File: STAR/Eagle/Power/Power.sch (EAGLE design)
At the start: 24 parts, among them J1 J30J-9J30, T1 750311838, U1 LT8300, U2 LT8330

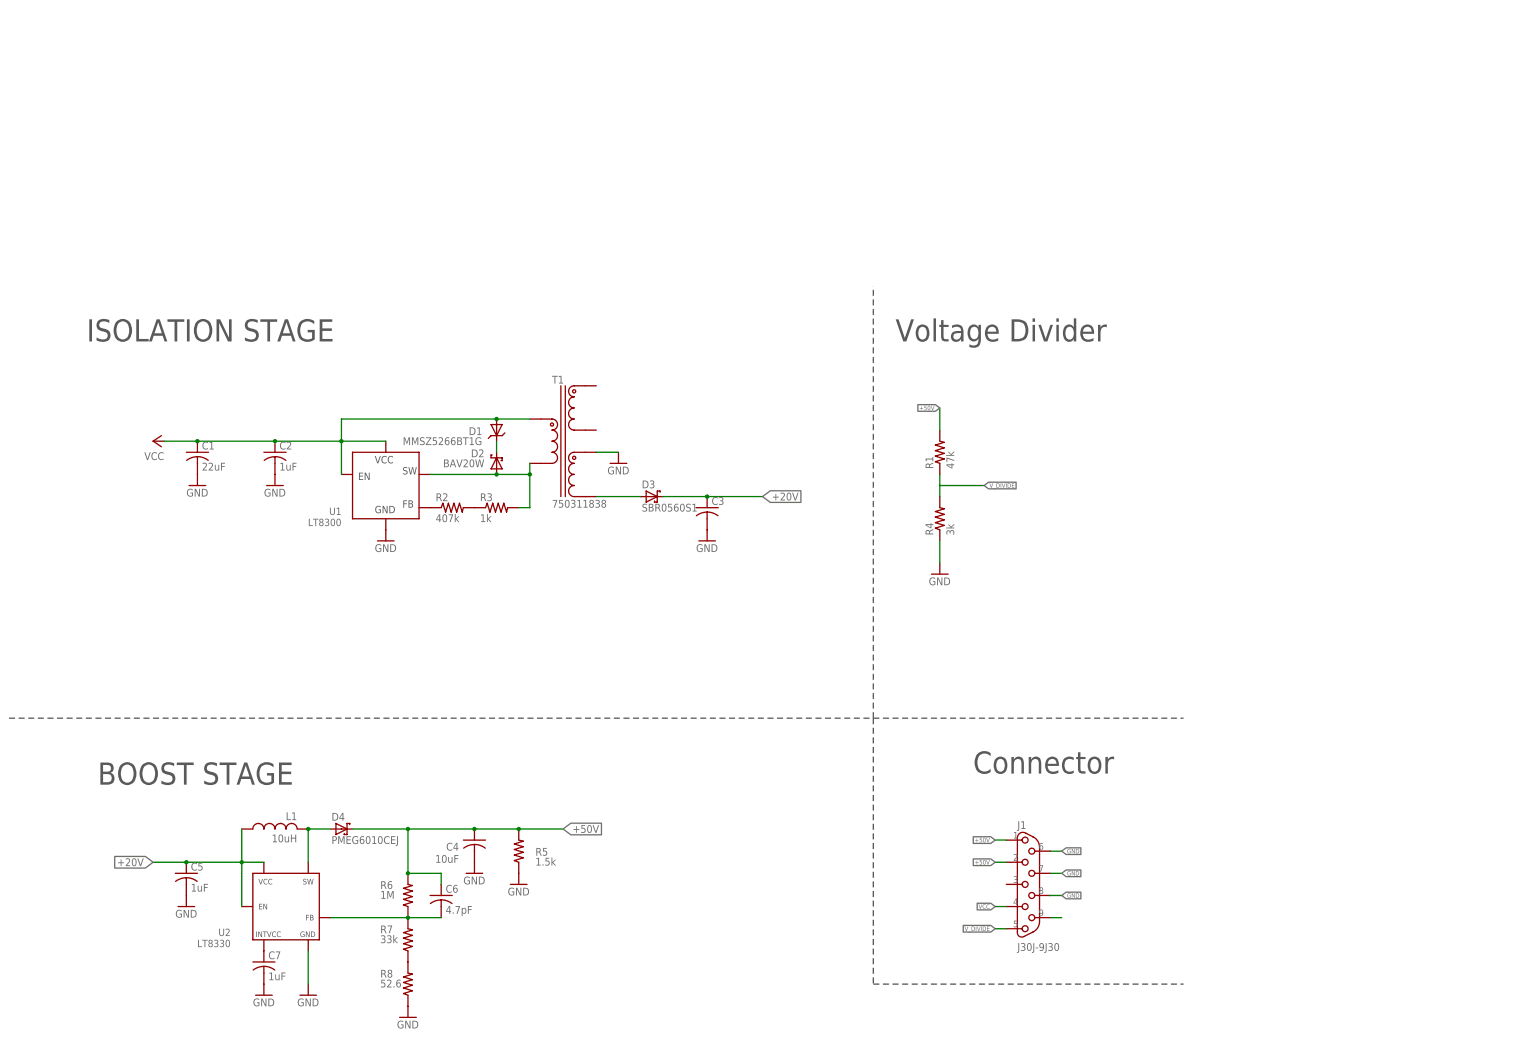
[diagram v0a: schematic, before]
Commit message: Power Board
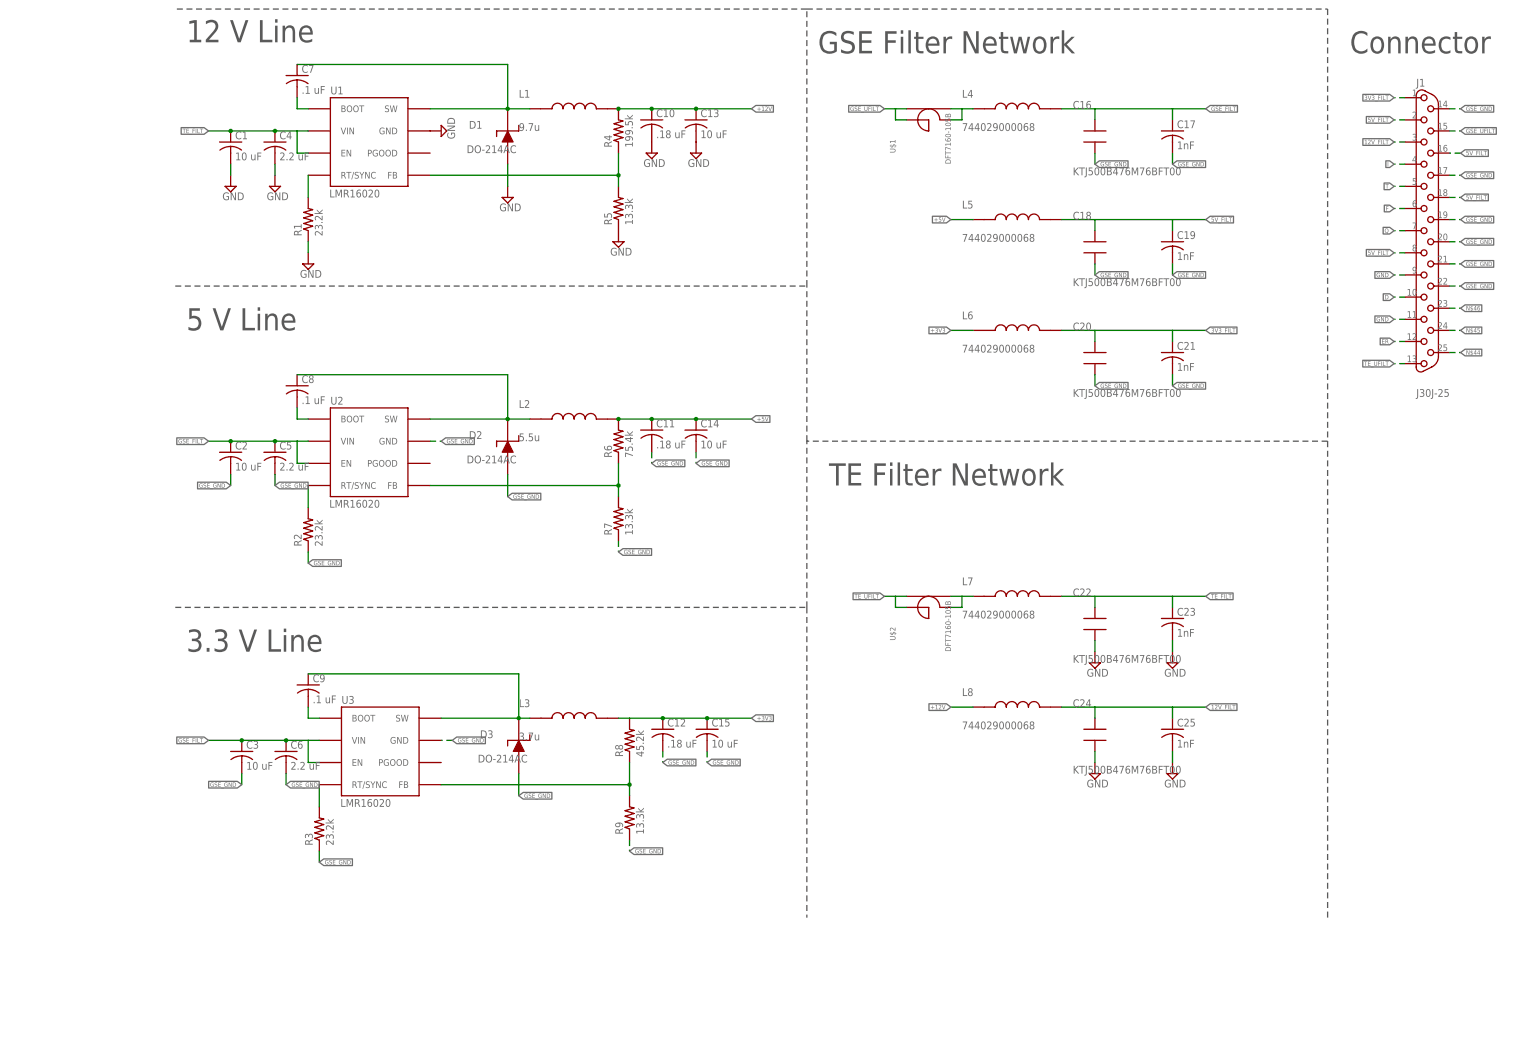
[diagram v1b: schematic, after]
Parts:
- removed D4: PMEG6010CEJ, AR_diode:SCHOTTKYSOD323
- removed T1: 750311838, AR_transformer:750311838
- added C10, C11, C12: .18 uF, resistor:C-USC0603
- added C13, C14, C15: 10 uF, resistor:C-USC0603
- added C16, C18, C20, C22, C24: KTJ500B476M76BFT00, Filtering:KTJ500B476M76BFT00
- added C17, C19, C21, C23, C25: 1nF, resistor:C-USC0603
- added C8, C9: .1 uF, resistor:C-USC0603
- added L2: 5.5u, Filtering:744325550
- added L3: 3.7u, Power:7443551370
- added L4, L5, L6, L7, L8: 744029000068, Filtering:744029000068
- added R9: 13.3k, resistor:R-US_R0603
- added U$1, U$2: DFT7160-105B, Filtering:DFT7160-105B
- added U3: LMR16020, HASP:LMR16020
- C1: value 22uF -> 10 uF; device AR_passives:CAPACITORC3025 -> resistor:C-USC1210
- C2: value 1uF -> 10 uF; device AR_passives:CAPACITORC0603 -> resistor:C-USC1210
- C3: value (none) -> 10 uF
- C4: value 10uF -> 2.2 uF; device AR_passives:CAPACITOR2-J-LEAD -> resistor:C-USC1210
- C5: value 1uF -> 2.2 uF; device AR_passives:CAPACITORC0603 -> resistor:C-USC1210
- C6: value 4.7pF -> 2.2 uF; device AR_passives:CAPACITORC0603 -> resistor:C-USC1210
- C7: value 1uF -> .1 uF; device AR_passives:CAPACITORC0603 -> resistor:C-USC0603
- D1: value MMSZ5266BT1G -> DO-214AC; device AR_diode:ZENERSOD123 -> HASP:DO-214AC
- D2: value BAV20W -> DO-214AC; device AR_diode:SCHOTTKYSOD323 -> HASP:DO-214AC
- D3: value SBR0560S1 -> DO-214AC; device AR_diode:SCHOTTKYSOD123 -> HASP:DO-214AC
- J1: value J30J-9J30 -> J30J-25; device CM_J30J:J30J-9J30 -> CM_J30J:J30J-25
- L1: value 10uH -> 9.7u; device AR_passives:INDUCTORPQ2614 -> Power:744314101
- R1: value 47k -> 23.2k; device resistor:R-US_R2512 -> resistor:R-US_R0603
- R2: value 407k -> 23.2k
- R3: value 1k -> 23.2k
- R4: value 3k -> 199.5k; device resistor:R-US_R2512 -> resistor:R-US_R0603
- R5: value 1.5k -> 13.3k; device resistor:R-US_R2512 -> resistor:R-US_R0603
- R6: value 1M -> 75.4k
- R7: value 33k -> 13.3k
- R8: value 52.6 -> 45.2k
- U1: value LT8300 -> LMR16020; device AR_IC:LT8300 -> HASP:LMR16020
- U2: value LT8330 -> LMR16020; device AR_IC:LT8330 -> HASP:LMR16020
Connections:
- removed net +20V: C3.1, C5.1, D3.C, L1.1, U2.EN, U2.VCC
- removed net +50V: C4.1, C6.1, D4.C, J1.1, J1.2, R1.2, R5.2, R6.2
- removed net N$11: R7.1, R8.2
- removed net VCC: C1.1, C2.1, D1.A, J1.4, T1.PA, U1.EN, U1.VCC
- removed net V_DIVIDE: J1.5, R1.1, R4.2
- new net +12V: C10.1, C13.1, L1.P$2, L8.P$1, R4.2
- new net +3V3: C12.1, C15.1, L3.P$2, L6.P$1, R8.2
- new net +5V: C11.1, C14.1, L2.P$2, L5.P$1, R6.2
- new net 12V_FILT: C24.P$1, C25.1, J1.3, L8.P$2
- new net 3V3_FILT: C20.P$1, C21.1, J1.1, L6.P$2
- new net 5V_FILT: C18.P$1, C19.1, J1.16, J1.18, J1.2, J1.8, L5.P$2
- new net D: J1.10
- new net ER: J1.12
- new net F: J1.6
- new net GSE_FILT: C16.P$1, C17.1, C2.1, C3.1, C5.1, C6.1, L4.P$2, U2.EN, U2.VIN, U3.EN, U3.VIN
- new net GSE_GND: C11.2, C12.2, C14.2, C15.2, C16.P$2, C17.2, C18.P$2, C19.2, C2.2, C20.P$2, C21.2, C3.2, C5.2, C6.2, D2.P$1, D3.P$1, J1.14, J1.17, J1.19, J1.20, J1.21, J1.22, R2.1, R3.1, R7.1, R9.1, U2.GND, U3.GND
- new net GSE_UFILT: J1.15, U$1.P$1, U$1.P$3
- new net I: J1.4
- new net N$14: C7.1, D1.P$2, L1.P$1, U1.SW
- new net N$27: R4.1, R5.2, U1.FB
- new net N$28: L4.P$1, U$1.P$2, U$1.P$4
- new net N$29: L7.P$1, U$2.P$2, U$2.P$4
- new net N$44: J1.25
- new net N$45: J1.24
- new net N$46: J1.23
- new net N$8: R8.1, R9.2, U3.FB
- new net Q: J1.7
- new net T: J1.5
- new net TE_FILT: C1.1, C22.P$1, C23.1, C4.1, L7.P$2, U1.EN, U1.VIN
- new net TE_UFILT: J1.13, U$2.P$1, U$2.P$3
- net GND: now also C10.2, C13.2, C22.P$2, C23.2, C24.P$2, C25.2, D1.P$1, J1.11, J1.9, R1.1; no longer C2.2, C3.2, C5.2, C7.2, J1.6, J1.7, R4.1, R8.1, T1.S2A, U2.GND
- net N$1: now also R3.2, U3.RT/SYNC; no longer D1.C, D2.C
- net N$10: now also C7.2, U1.BOOT; no longer J1.9
- net N$2: now also C9.1, D3.P$2, L3.P$1, U3.SW; no longer R2.1, U1.FB
- net N$3: now also U2.RT/SYNC; no longer R3.1
- net N$4: now also C8.2, U2.BOOT; no longer D2.A, R3.2, T1.PB, U1.SW
- net N$5: now also C8.1, D2.P$2, L2.P$1, U2.SW; no longer D3.A, T1.S2B
- net N$6: now also C9.2, U3.BOOT; no longer C7.1, U2.INTVCC
- net N$7: now also R1.2, U1.RT/SYNC; no longer D4.A, L1.2, U2.SW
- net N$9: no longer C6.2
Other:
- note added: "12 V Line"
- note added: "3.3 V Line"
- note added: "5 V Line"
- note added: "GSE Filter Network"
- note added: "TE Filter Network"
- note removed: "BOOST STAGE"
- note removed: "ISOLATION STAGE"
- note removed: "Voltage Divider"
- moved on the sheet: C1, C2, C3, C4, C5, C6, C7, R1, R2, R3, R4, R5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
